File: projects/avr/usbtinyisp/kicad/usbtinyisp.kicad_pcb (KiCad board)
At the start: 2 copper layers, 76.2 x 38.1 mm, 19 parts, among them J1 USB_2, P1 CONN_6, SW1 SWITCH_INV, U1 ATTINY2313-20PU, X1 CRYSTAL

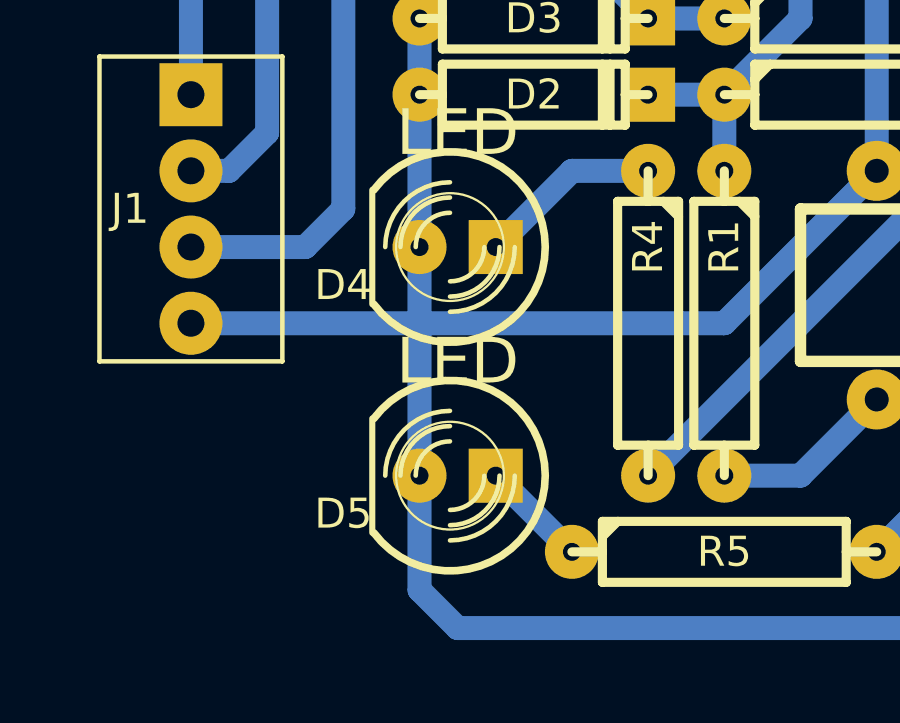
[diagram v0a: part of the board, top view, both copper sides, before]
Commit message: update kicad files
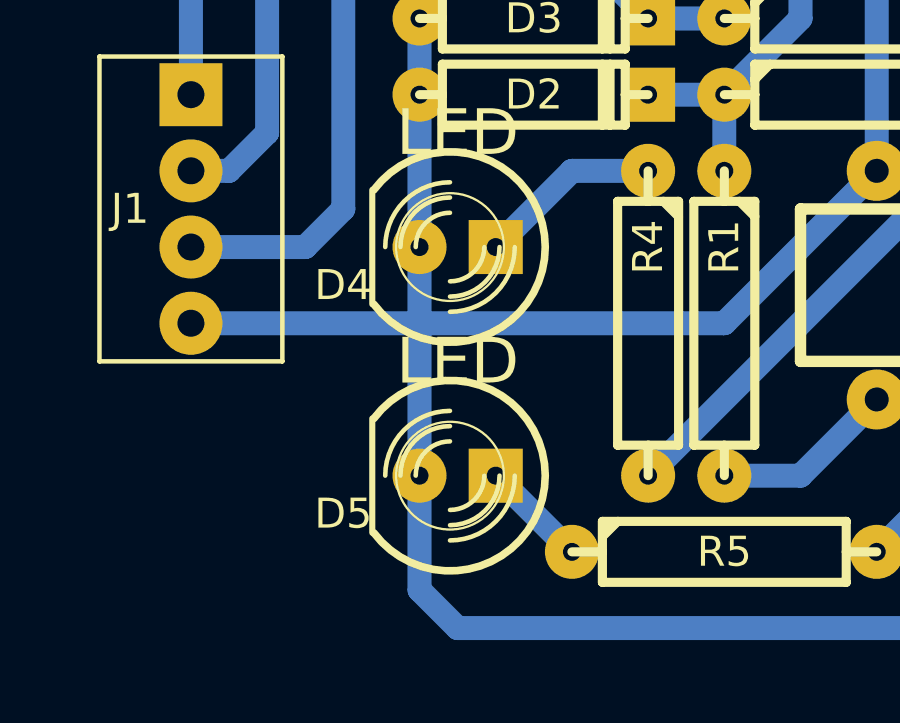
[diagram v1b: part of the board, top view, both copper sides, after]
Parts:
- C1, C2: footprint kicad:C2 -> common:C2
- C3: footprint kicad:CP_5x11mm -> common:CP_5x11mm
- D2, D3: footprint kicad:D3 -> common:D3
- D4, D5: footprint kicad:LED-5MM -> common:LED-5MM
- J1: footprint kicad:USB4 -> common:USB4
- JP1: footprint kicad:BR2 -> common:BR2
- P1: footprint kicad:PIN_ARRAY_6X1 -> common:PIN_ARRAY_6X1
- R1, R2, R3, R4, R5, R6: footprint kicad:R4 -> common:R4
- SW1: footprint kicad:MICROSWITCH_SPST -> common:MICROSWITCH_SPST
- U1: footprint kicad:DIP-20__300 -> common:DIP-20__300
- X1: footprint kicad:QUARTZ -> common:QUARTZ
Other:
- net class Default removed
